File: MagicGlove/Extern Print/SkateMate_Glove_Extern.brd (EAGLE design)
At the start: 43 x 27 mm, 42 parts, among them IC1 BU33TD3WG, IC2 LMV321M5, U2 ATMEGA328PB-AU

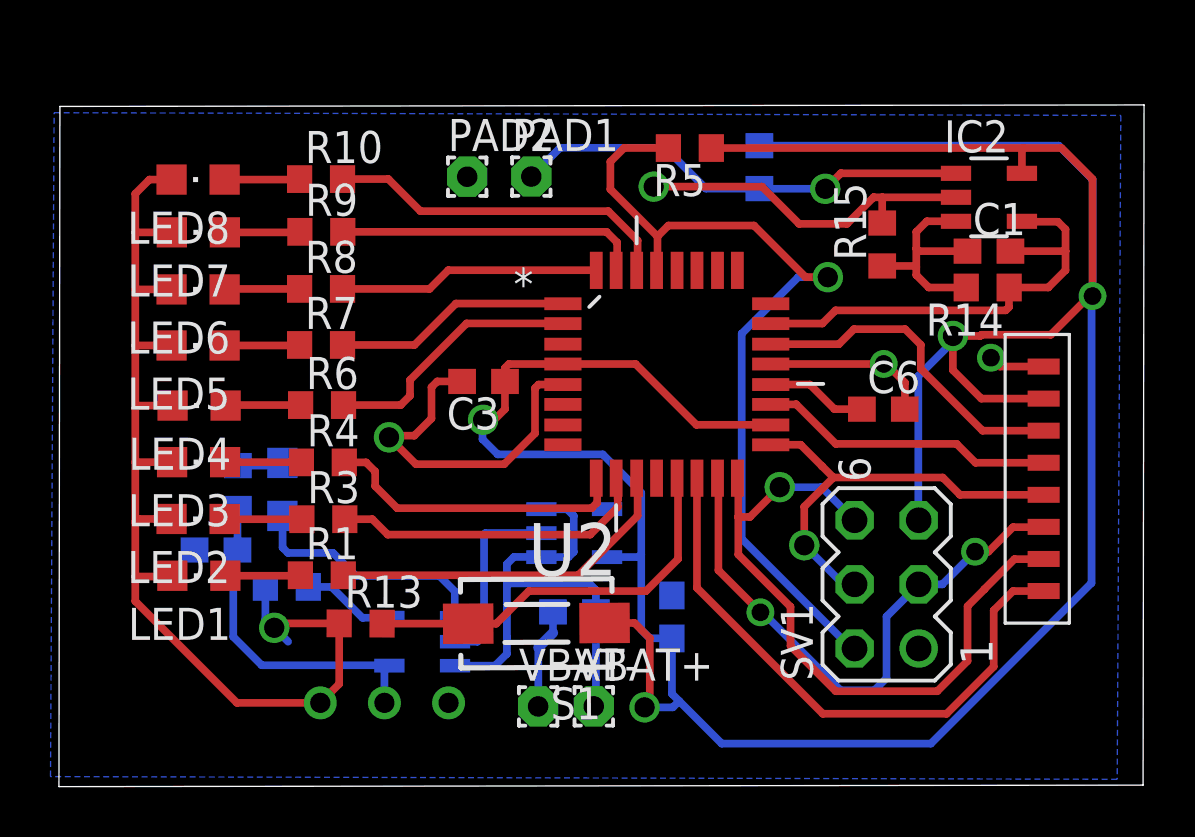
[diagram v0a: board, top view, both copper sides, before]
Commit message: Backup commit.
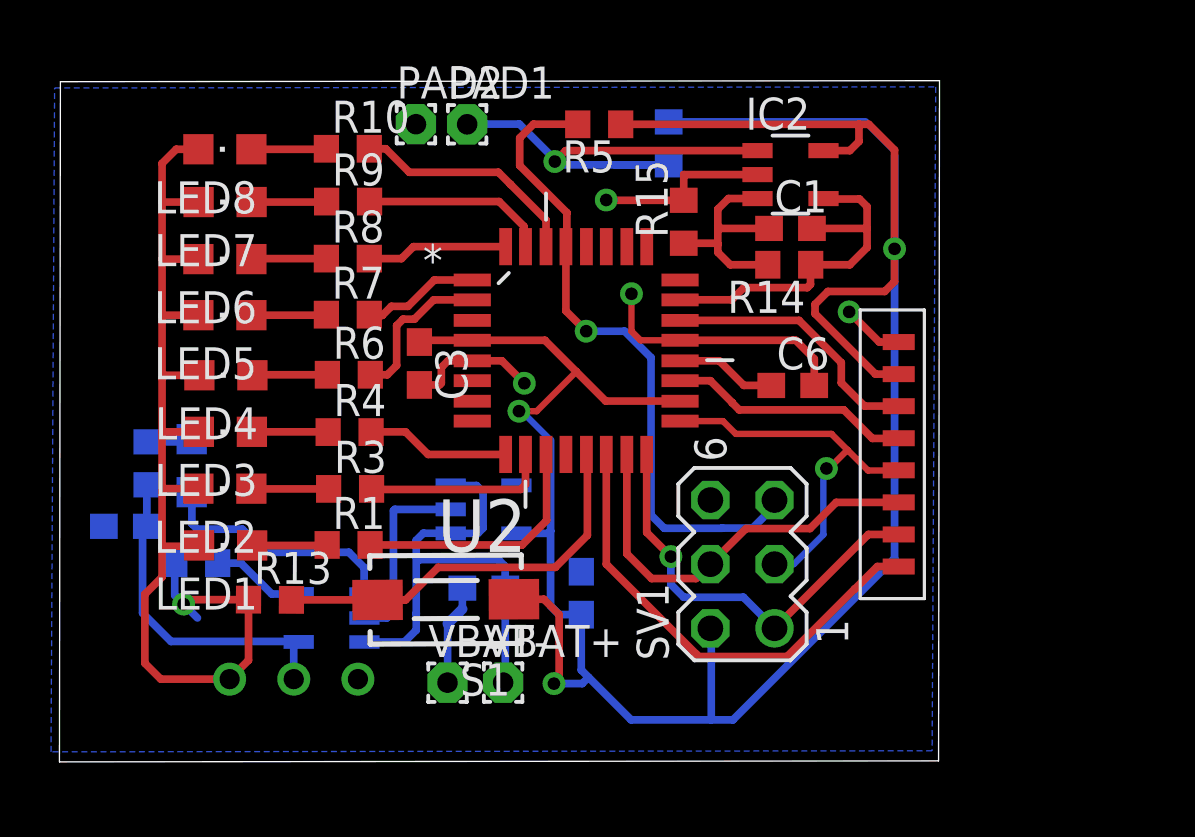
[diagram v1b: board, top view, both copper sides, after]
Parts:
- moved R14 7.91 mm to (28.9, 19.7)
- moved C1 7.91 mm to (28.9, 21.1)
- moved IC2 7.91 mm to (28.9, 23.3)
- moved R15 7.91 mm to (24.7, 21.4)
- moved U$2 5.82 mm to (34.2, 12.2)
- moved SV1 5.77 mm to (27.0, 7.83)
- moved R13 3.71 mm to (8.33, 6.42)
- moved LED9 3.71 mm to (5.23, 11.7)
- moved R11 3.71 mm to (5.41, 7.87)
- moved R5 3.71 mm to (21.4, 25.2)
- moved U$1 3.71 mm to (10.8, 5.70)
- moved C9 3.71 mm to (2.61, 9.33)
- moved C7 3.71 mm to (20.7, 6.68)
- moved C8 3.71 mm to (16.8, 6.88)
- moved IC1 3.71 mm to (16.8, 10.0)
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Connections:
- net +3V3: now also SV1.2; no longer SV1.5
- net GND: now also SV1.6; no longer SV1.1
- net MISO: now also SV1.1; no longer SV1.6
- net MOSI: now also SV1.4; no longer SV1.3
- net RESETICSP: now also SV1.5; no longer SV1.2
- net SCK: now also SV1.3; no longer SV1.4
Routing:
- net +3V3: track 129.4 -> 105.9 mm, vias 4 -> 3
- net GND: track 94.5 -> 80.9 mm
- net MISO: track 27.6 -> 16.8 mm
- net RESETICSP: track 34.2 -> 26.3 mm
- net N$15: track 12.2 -> 5.70 mm
- net MOSI: track 22.6 -> 16.4 mm, vias 2 -> 0
- net N$13: track 13.5 -> 7.38 mm
- net N$19: track 12.2 -> 7.35 mm
- net N$18: track 10.4 -> 5.59 mm
- net N$17: track 9.42 -> 4.68 mm
- net N$20: track 13.9 -> 9.25 mm
- net IRQ: track 23.5 -> 18.9 mm
- net N$14: track 19.0 -> 14.7 mm
- net N$16: track 10.4 -> 6.19 mm
- net N$12: track 14.1 -> 10.0 mm
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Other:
- board size 43 x 27 mm -> 34.9 x 27 mm
